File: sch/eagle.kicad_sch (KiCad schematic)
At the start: 4 parts, among them U1 RP2040, U2 MPU-6050, U3 BMP280

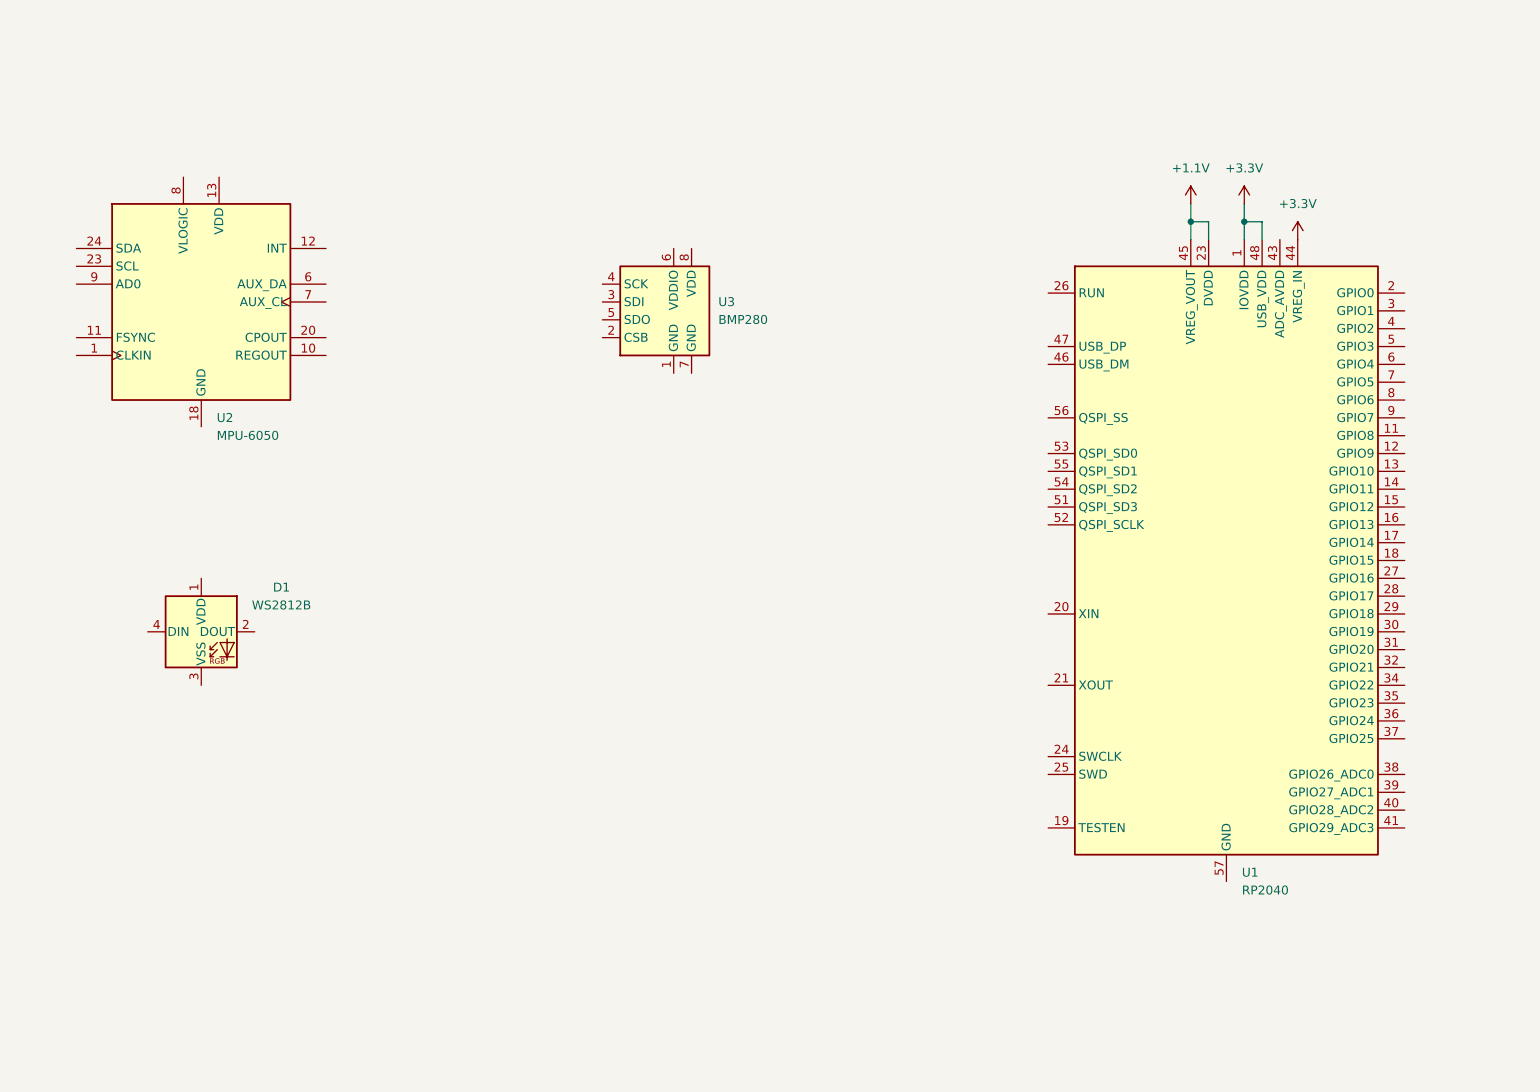
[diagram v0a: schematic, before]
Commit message: Added to schematic
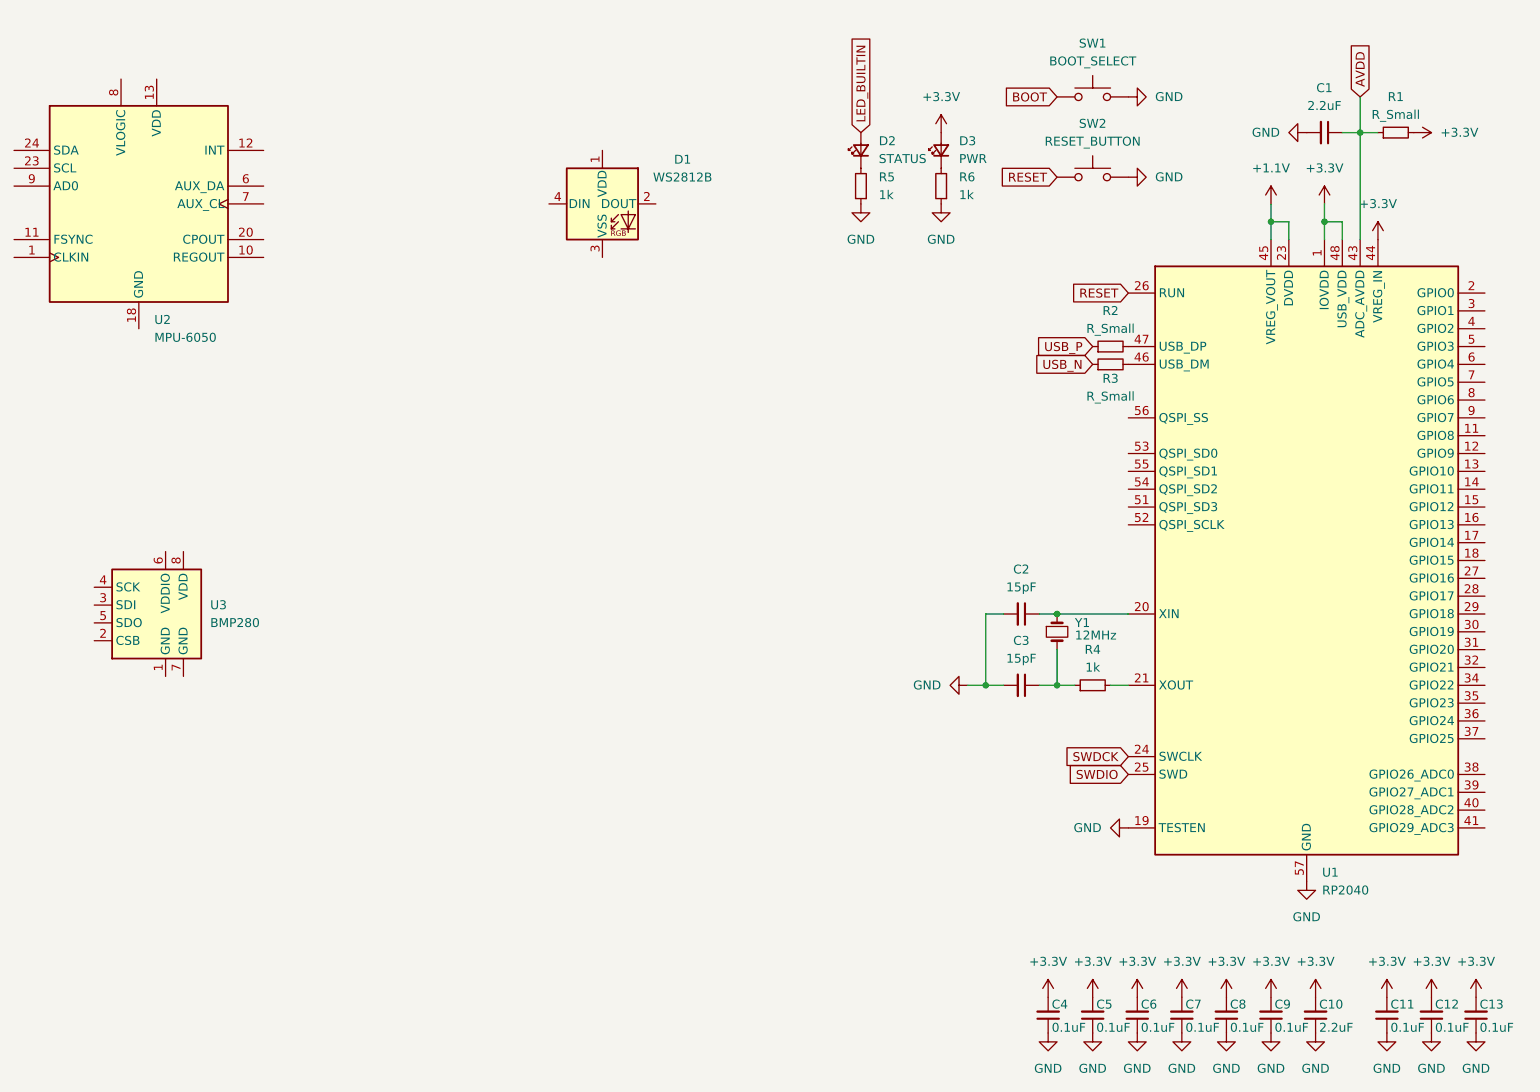
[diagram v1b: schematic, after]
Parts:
- added C1, C10: 2.2uF, symbol Device:C_Small
- added C11, C12, C13, C4, C5, C6, C7, C8, C9: 0.1uF, symbol Device:C_Small
- added C2, C3: 15pF, symbol Device:C_Small
- added D2: STATUS, symbol Device:LED_Small
- added D3: PWR, symbol Device:LED_Small
- added R1, R2, R3: R_Small, symbol Device:R_Small
- added R4, R5, R6: 1k, symbol Device:R_Small
- added SW1: BOOT_SELECT, symbol Switch:SW_Push
- added SW2: RESET_BUTTON, symbol Switch:SW_Push
- added Y1: 12MHz, symbol Device:Crystal_Small
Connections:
- net +3.3V: now also C10.2, C11.2, C12.2, C13.2, C4.2, C5.2, C6.2, C7.2, C8.2, C9.2, D3.2 (A), R1.2
- net GND: now reaches U1.19 (TESTEN)
- net GND: now also U1.57 (GND), C1.2, C10.1, C11.1, C12.1, C13.1, C2.2, C3.2, C4.1, C5.1, C6.1, C7.1, C8.1, C9.1, R5.1, R6.1, SW1.2, SW2.2
- net at U1.20 (XIN): now also C2.1, Y1.1
- net at U1.21 (XOUT): now also R4.2
- net SWDCK: now reaches U1.24 (SWCLK)
- net SWDIO: now reaches U1.25 (SWD)
- net RESET: now reaches U1.26 (RUN)
- net RESET: now also SW2.1
- net AVDD: now reaches U1.43 (ADC_AVDD)
- net AVDD: now also C1.1, R1.1
- net at U1.46 (USB_DM): now also R3.2
- net at U1.47 (USB_DP): now also R2.2
- new net: C3.1, R4.1, Y1.2
- new net: D3.1 (K), R6.2
- new net: D2.1 (K), R5.2
- new net BOOT: SW1.1
- new net LED_BUILTIN: D2.2 (A)
- new net USB_N: R3.1
- new net USB_P: R2.1
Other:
- moved on the sheet: D1, U1, U2, U3
